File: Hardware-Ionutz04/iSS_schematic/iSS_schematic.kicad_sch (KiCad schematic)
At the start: 6 parts, among them U1 ACS37800KMACTR-030B3-I2C

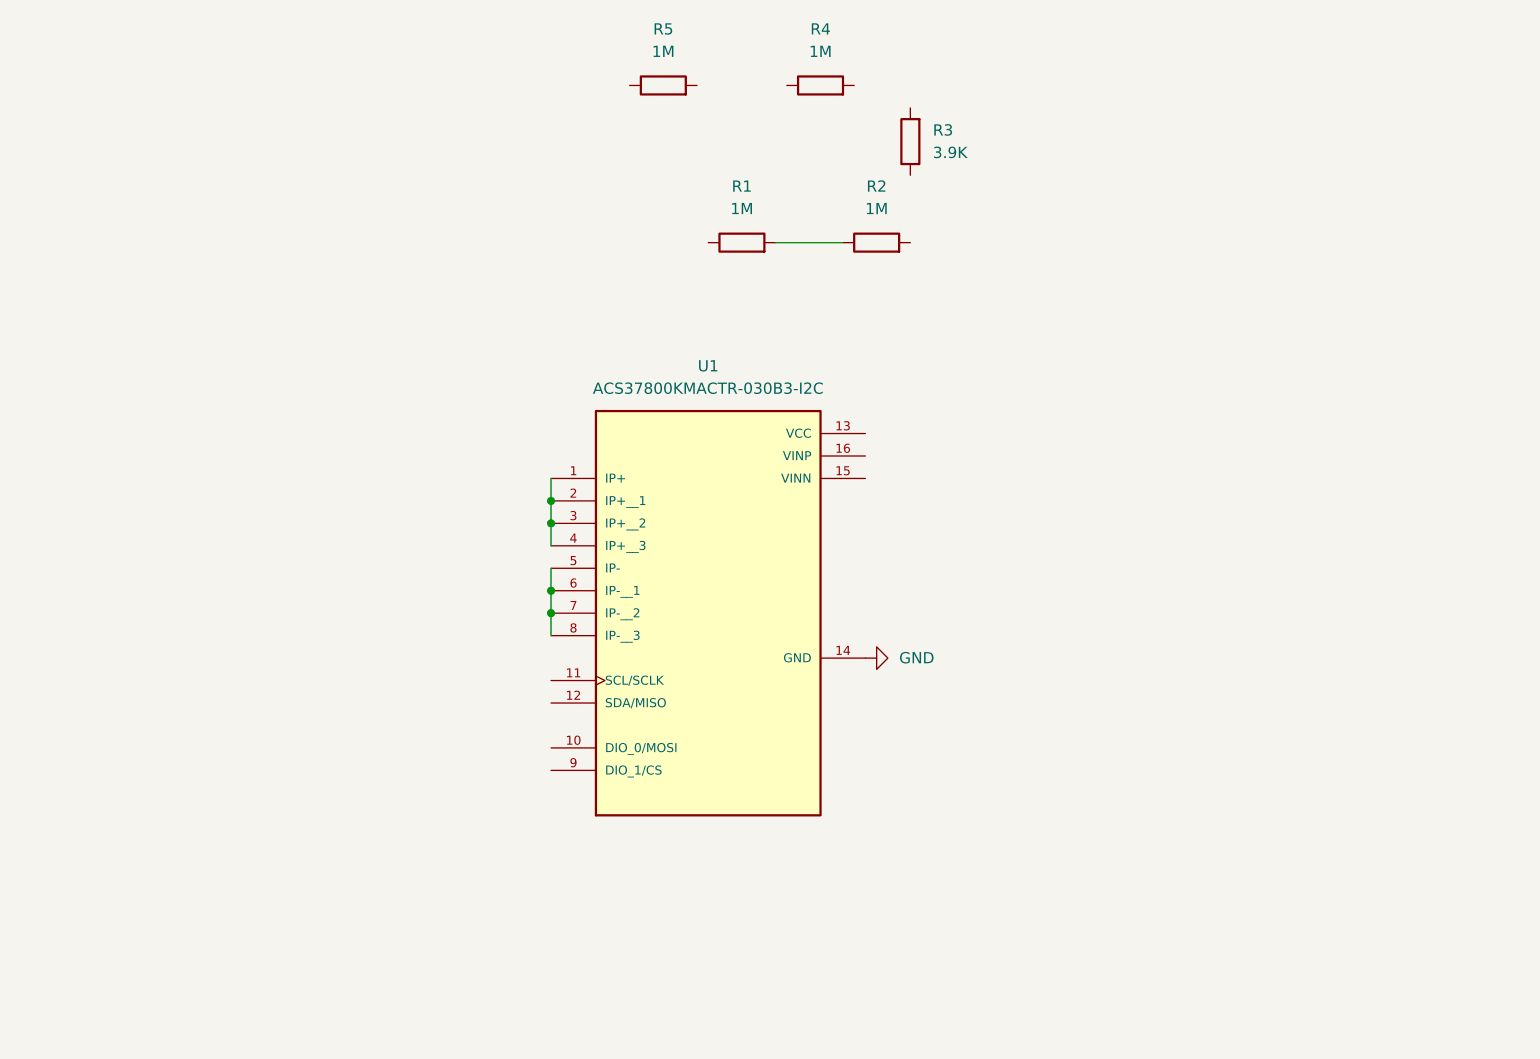
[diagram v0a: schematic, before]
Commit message: Beta commit on firmware side of the iSS
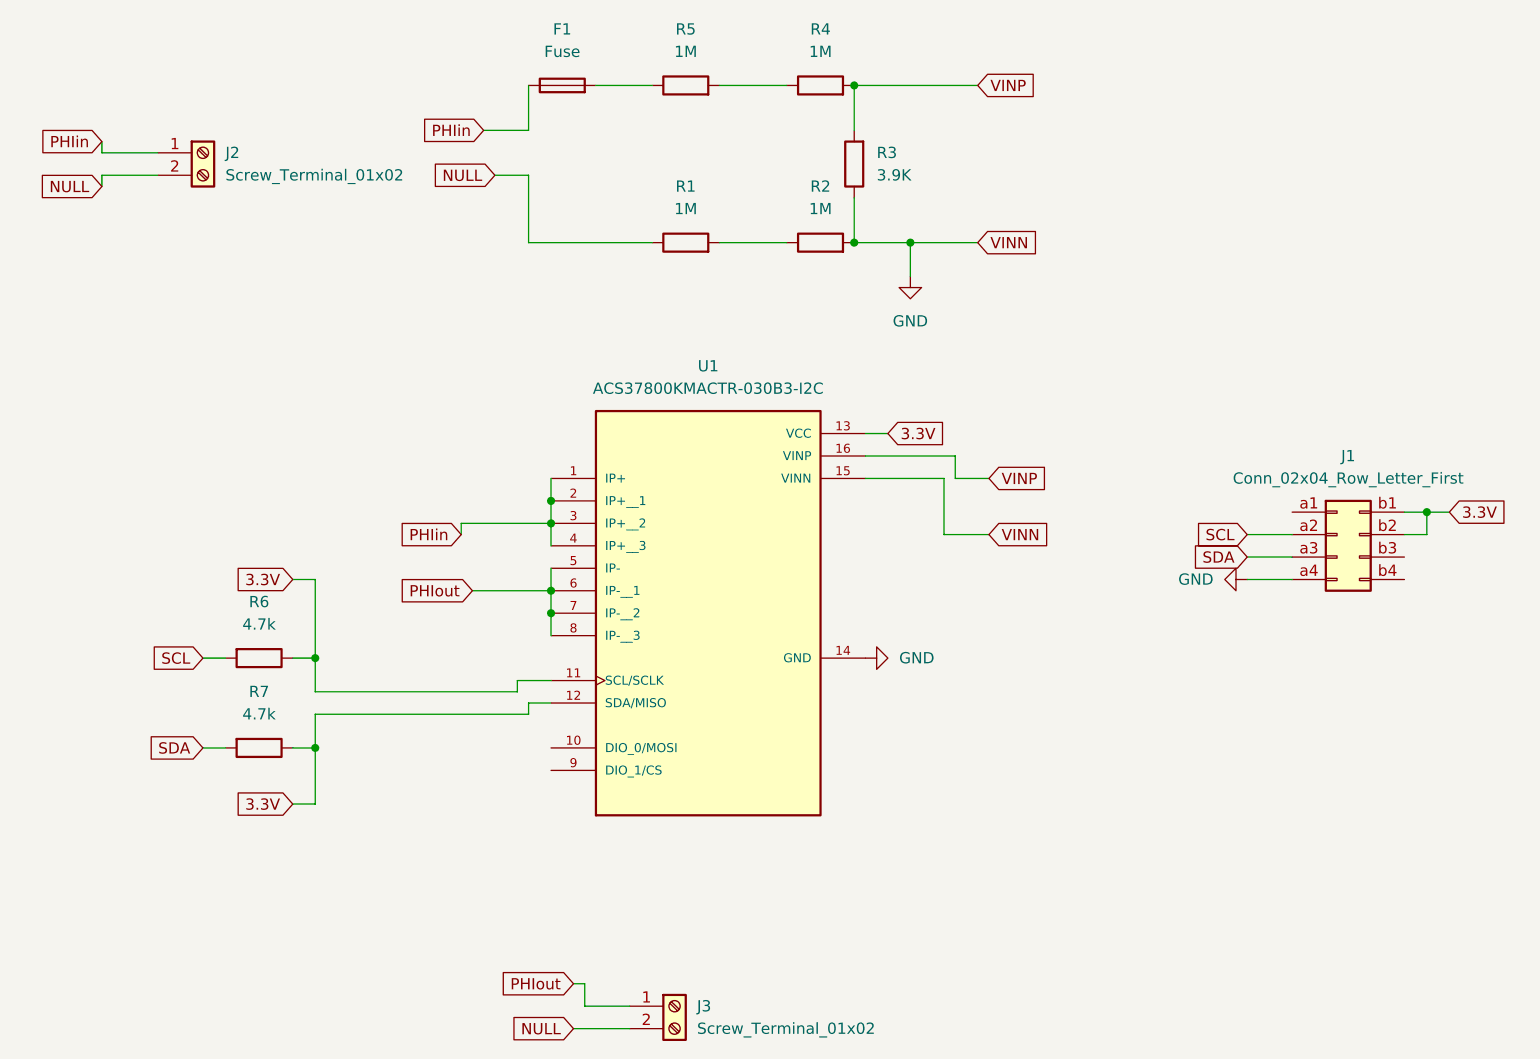
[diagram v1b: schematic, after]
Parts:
- added F1: Fuse, Fuse:Fuse_0603_1608Metric_Pad1.05x0.95mm_HandSolder, symbol Device:Fuse
- added J1: Conn_02x04_Row_Letter_First, Connector_PinHeader_2.54mm:PinHeader_2x04_P2.54mm_Vertical, symbol Connector_Generic:Conn_02x04_Row_Letter_First
- added J2, J3: Screw_Terminal_01x02, TerminalBlock_CUI:TerminalBlock_CUI_TB007-508-02_1x02_P5.08mm_Horizontal, symbol Connector:Screw_Terminal_01x02
- added R6, R7: 4.7k, Resistor_SMD:R_1206_3216Metric_Pad1.30x1.75mm_HandSolder, symbol Device:R
- R1, R2, R3, R4, R5: footprint (none) -> Resistor_SMD:R_1206_3216Metric_Pad1.30x1.75mm_HandSolder
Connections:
- net GND: now also R2.2, R3.1, U1.15 (VINN), J1.a4 (Pin_a4)
- net NULL: now reaches R1.1
- net NULL: now also J2.2 (Pin_2), J3.2 (Pin_2)
- net PHIin: now reaches U1.1 (IP+), U1.2 (IP+__1), U1.3 (IP+__2), U1.4 (IP+__3)
- net PHIin: now also F1.1, J2.1 (Pin_1)
- net 3.3V: now reaches U1.11 (SCL/SCLK)
- net 3.3V: now also U1.12 (SDA/MISO), U1.13 (VCC), J1.b1 (Pin_b1), J1.b2 (Pin_b2), R6.1, R7.1
- net VINP: now reaches U1.16 (VINP)
- net VINP: now also R3.2, R4.2
- net PHIout: now reaches U1.5 (IP-), U1.6 (IP-__1), U1.7 (IP-__2), U1.8 (IP-__3)
- net PHIout: now also J3.1 (Pin_1)
- net at R4.1: now also R5.2
- net at R5.1: now also F1.2
- new net SCL: J1.a2 (Pin_a2), R6.2
- new net SDA: J1.a3 (Pin_a3), R7.2
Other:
- moved on the sheet: R1, R2, R3, R5
